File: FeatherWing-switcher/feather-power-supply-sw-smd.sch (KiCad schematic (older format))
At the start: 24 parts, among them J1 5.08mm, J2 Conn_01x12, J3 Conn_01x16, U1 TPS5405DR

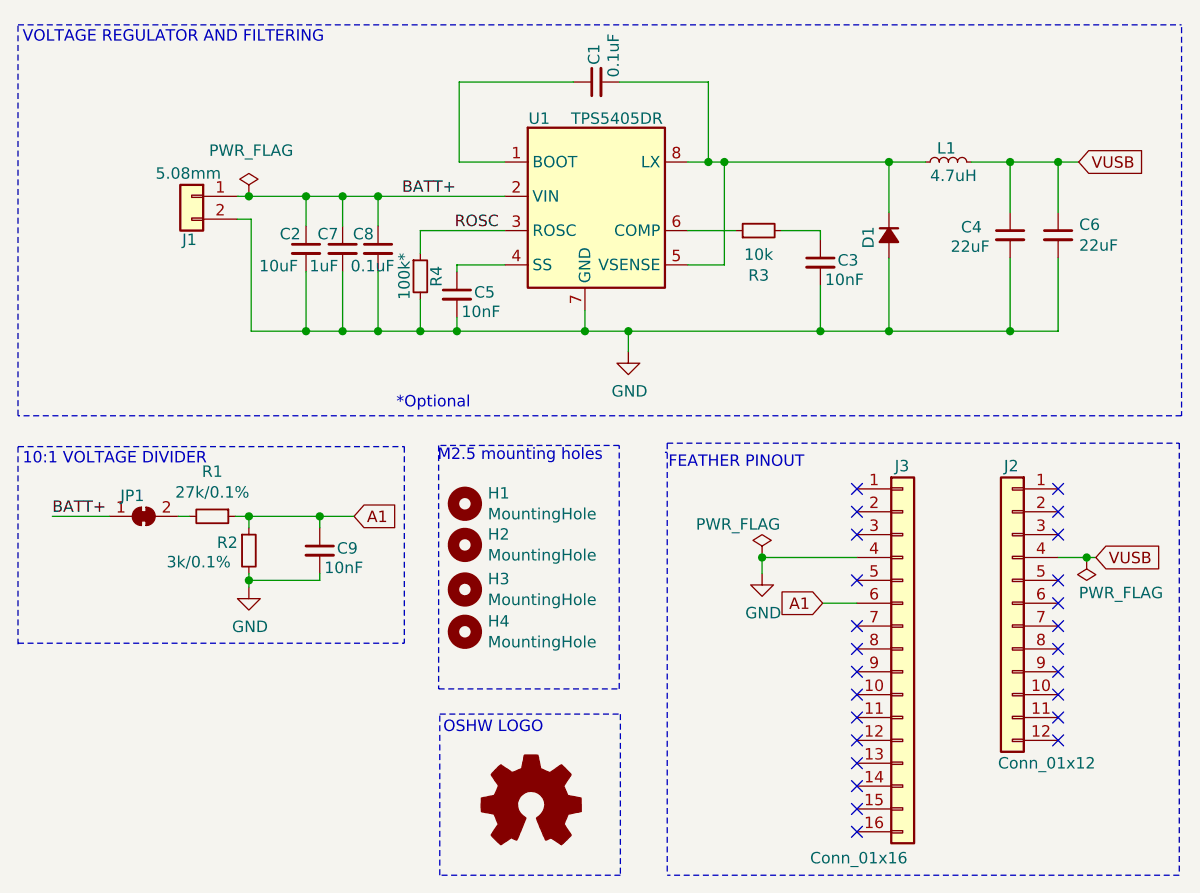
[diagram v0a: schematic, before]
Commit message: update mounting holes
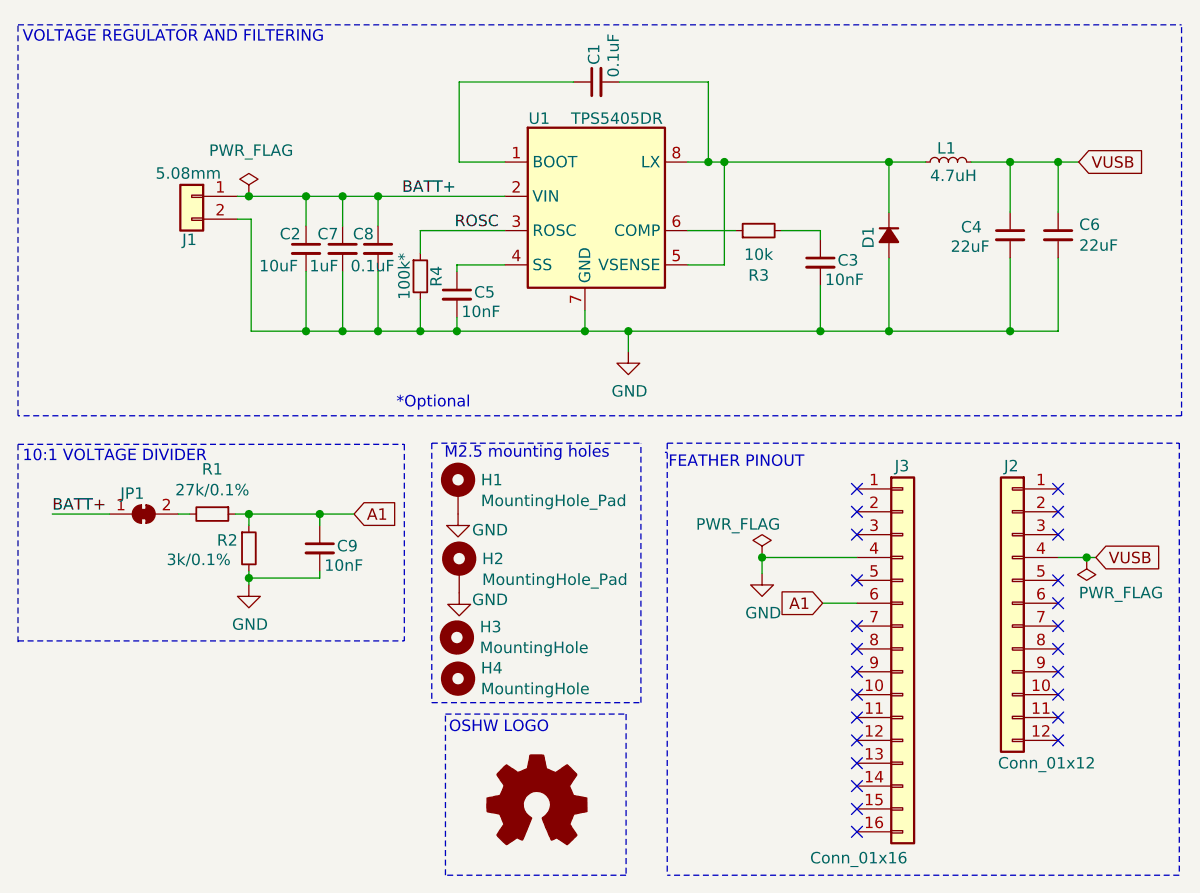
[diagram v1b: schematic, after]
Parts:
- removed H1, H2: MountingHole, MountingHole:MountingHole_2.7mm_M2.5, symbol Mechanical:MountingHole
- added H1, H2: MountingHole_Pad, MountingHole:MountingHole_2.5mm_Pad, symbol Mechanical:MountingHole_Pad
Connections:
- net GND: now also H1.1, H2.1
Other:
- moved on the sheet: H3, H4
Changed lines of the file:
@@
 $EndComp
 Connection ~ 6325 3900
-Text Label 3220 3720 0    50   ~ 0
+Text Label 3220 3710 0    50   ~ 0
 BATT+
-Text GLabel 4540 3720 2    50   Input ~ 0
+Text GLabel 4540 3710 2    50   Input ~ 0
 A1
 Text GLabel 6590 4100 0    50   Input ~ 0
@@
 	5910 3400 5910 5290
 Wire Notes Line
-	4760 3415 4760 4275
+	4760 3405 4760 4265
 Wire Notes Line
 	8160 1580 8160 3280
@@
 Wire Wire Line
 	4490 2910 4645 2910
-$Comp
-L Mechanical:MountingHole H1
-U 1 1 5F4DCA7B
-P 5025 3665
-F 0 "H1" H 5125 3711 50  0000 L CNN
-F 1 "MountingHole" H 5125 3620 50  0000 L CNN
-F 2 "MountingHole:MountingHole_2.7mm_M2.5" H 5025 3665 50  0001 C CNN
-F 3 "~" H 5025 3665 50  0001 C CNN
-	1    5025 3665
-	1    0    0    -1
-$EndComp
-$Comp
-L Mechanical:MountingHole H2
-U 1 1 5F4E3BF8
-P 5025 3845
-F 0 "H2" H 5125 3891 50  0000 L CNN
-F 1 "MountingHole" H 5125 3800 50  0000 L CNN
-F 2 "MountingHole:MountingHole_2.7mm_M2.5" H 5025 3845 50  0001 C CNN
-F 3 "~" H 5025 3845 50  0001 C CNN
-	1    5025 3845
-	1    0    0    -1
-$EndComp
-$Comp
-L Mechanical:MountingHole H3
-U 1 1 5F4E3ED4
-P 5025 4040
-F 0 "H3" H 5125 4086 50  0000 L CNN
-F 1 "MountingHole" H 5125 3995 50  0000 L CNN
-F 2 "MountingHole:MountingHole_2.7mm_M2.5" H 5025 4040 50  0001 C CNN
-F 3 "~" H 5025 4040 50  0001 C CNN
-	1    5025 4040
-	1    0    0    -1
-$EndComp
-$Comp
-L Mechanical:MountingHole H4
-U 1 1 5F4E4234
-P 5025 4225
-F 0 "H4" H 5125 4271 50  0000 L CNN
-F 1 "MountingHole" H 5125 4180 50  0000 L CNN
-F 2 "MountingHole:MountingHole_2.7mm_M2.5" H 5025 4225 50  0001 C CNN
-F 3 "~" H 5025 4225 50  0001 C CNN
-	1    5025 4225
-	1    0    0    -1
-$EndComp
-Wire Notes Line
-	4910 4475 5700 4475
-Wire Notes Line
-	5700 4475 5700 3410
-Wire Notes Line
-	5700 3410 4910 3410
-Wire Notes Line
-	4910 3410 4910 4475
-Text Notes 4905 3485 0    50   ~ 0
+Text Notes 4935 3475 0    50   ~ 0
 M2.5 mounting holes
 Wire Wire Line
-	3220 3720 3470 3720
-Wire Notes Line
-	3070 4275 4760 4275
-Wire Notes Line
-	3070 3415 4760 3415
-Wire Notes Line
-	3070 3415 3070 4280
+	3220 3710 3470 3710
+Wire Notes Line
+	3070 4265 4760 4265
+Wire Notes Line
+	3070 3405 4760 3405
+Wire Notes Line
+	3070 3405 3070 4270
 $Comp
 L Jumper:SolderJumper_2_Bridged JP1
 U 1 1 5F4E9F72
-P 3620 3720
-F 0 "JP1" H 3570 3810 50  0000 C CNN
-F 1 "SolderJumper_2_Bridged" H 3285 3630 50  0001 C CNN
-F 2 "Jumper:SolderJumper-2_P1.3mm_Bridged_RoundedPad1.0x1.5mm" H 3620 3720 50  0001 C CNN
-F 3 "~" H 3620 3720 50  0001 C CNN
-	1    3620 3720
-	1    0    0    -1
-$EndComp
-Text Notes 3090 3500 0    50   ~ 0
+P 3620 3710
+F 0 "JP1" H 3570 3800 50  0000 C CNN
+F 1 "SolderJumper_2_Bridged" H 3285 3620 50  0001 C CNN
+F 2 "Jumper:SolderJumper-2_P1.3mm_Bridged_RoundedPad1.0x1.5mm" H 3620 3710 50  0001 C CNN
+F 3 "~" H 3620 3710 50  0001 C CNN
+	1    3620 3710
+	1    0    0    -1
+$EndComp
+Text Notes 3090 3490 0    50   ~ 0
 10:1 VOLTAGE DIVIDER
 Wire Wire Line
-	4080 4030 4080 4000
-Wire Wire Line
-	4080 3720 4080 3770
+	4080 4020 4080 3990
+Wire Wire Line
+	4080 3710 4080 3760
 $Comp
 L power:GND #PWR02
 U 1 1 5F4755CE
-P 4080 4030
-F 0 "#PWR02" H 4080 3780 50  0001 C CNN
-F 1 "GND" H 4085 3857 50  0000 C CNN
-F 2 "" H 4080 4030 50  0001 C CNN
-F 3 "" H 4080 4030 50  0001 C CNN
-	1    4080 4030
+P 4080 4020
+F 0 "#PWR02" H 4080 3770 50  0001 C CNN
+F 1 "GND" H 4085 3847 50  0000 C CNN
+F 2 "" H 4080 4020 50  0001 C CNN
+F 3 "" H 4080 4020 50  0001 C CNN
+	1    4080 4020
 	1    0    0    -1
 $EndComp
@@
 L Device:R_Small R1
 U 1 1 5F47540B
-P 3920 3720
-F 0 "R1" V 3724 3720 50  0000 C CNN
-F 1 "27k/0.1%" V 3815 3720 50  0000 C CNN
-F 2 "Resistor_SMD:R_0603_1608Metric_Pad1.05x0.95mm_HandSolder" H 3920 3720 50  0001 C CNN
-F 3 "~" H 3920 3720 50  0001 C CNN
-F 4 "‎P20138CT-ND‎" V 3920 3720 50  0001 C CNN "DigiKey_PN"
-	1    3920 3720
+P 3920 3710
+F 0 "R1" V 3724 3710 50  0000 C CNN
+F 1 "27k/0.1%" V 3815 3710 50  0000 C CNN
+F 2 "Resistor_SMD:R_0603_1608Metric_Pad1.05x0.95mm_HandSolder" H 3920 3710 50  0001 C CNN
+F 3 "~" H 3920 3710 50  0001 C CNN
+F 4 "‎P20138CT-ND‎" V 3920 3710 50  0001 C CNN "DigiKey_PN"
+	1    3920 3710
 	0    1    1    0
 $EndComp
@@
 L Device:R_Small R2
 U 1 1 5F475325
-P 4080 3870
-F 0 "R2" H 3940 3905 50  0000 L CNN
-F 1 "3k/0.1%" H 3720 3820 50  0000 L CNN
-F 2 "Resistor_SMD:R_0603_1608Metric_Pad1.05x0.95mm_HandSolder" H 4080 3870 50  0001 C CNN
-F 3 "~" H 4080 3870 50  0001 C CNN
-F 4 "P20072CT-ND‎" H 4080 3870 50  0001 C CNN "DigiKey_PN"
-	1    4080 3870
+P 4080 3860
+F 0 "R2" H 3940 3895 50  0000 L CNN
+F 1 "3k/0.1%" H 3720 3810 50  0000 L CNN
+F 2 "Resistor_SMD:R_0603_1608Metric_Pad1.05x0.95mm_HandSolder" H 4080 3860 50  0001 C CNN
+F 3 "~" H 4080 3860 50  0001 C CNN
+F 4 "P20072CT-ND‎" H 4080 3860 50  0001 C CNN "DigiKey_PN"
+	1    4080 3860
 	1    0    0    -1
 $EndComp
@@
 $EndComp
 Wire Wire Line
-	3770 3720 3820 3720
+	3770 3710 3820 3710
 $Comp
 L Device:C_Small C9
 U 1 1 5F52B2E4
-P 4390 3870
-F 0 "C9" H 4465 3880 50  0000 L CNN
-F 1 "10nF" H 4410 3795 50  0000 L CNN
-F 2 "Capacitor_SMD:C_0603_1608Metric_Pad1.05x0.95mm_HandSolder" H 4390 3870 50  0001 C CNN
-F 3 "~" H 4390 3870 50  0001 C CNN
-	1    4390 3870
-	1    0    0    -1
-$EndComp
-Wire Wire Line
-	4540 3720 4390 3720
-Connection ~ 4080 3720
-Wire Wire Line
-	4080 3720 4020 3720
-Wire Wire Line
-	4390 3770 4390 3720
-Connection ~ 4390 3720
-Wire Wire Line
-	4390 3720 4080 3720
-Wire Wire Line
-	4390 3970 4390 4000
-Wire Wire Line
-	4390 4000 4080 4000
-Connection ~ 4080 4000
-Wire Wire Line
-	4080 4000 4080 3970
-$Comp
-L Graphic:Logo_Open_Hardware_Small #LOGO?
+P 4390 3860
+F 0 "C9" H 4465 3870 50  0000 L CNN
+F 1 "10nF" H 4410 3785 50  0000 L CNN
+F 2 "Capacitor_SMD:C_0603_1608Metric_Pad1.05x0.95mm_HandSolder" H 4390 3860 50  0001 C CNN
+F 3 "~" H 4390 3860 50  0001 C CNN
+	1    4390 3860
+	1    0    0    -1
+$EndComp
+Wire Wire Line
+	4540 3710 4390 3710
+Connection ~ 4080 3710
+Wire Wire Line
+	4080 3710 4020 3710
+Wire Wire Line
+	4390 3760 4390 3710
+Connection ~ 4390 3710
+Wire Wire Line
+	4390 3710 4080 3710
+Wire Wire Line
+	4390 3960 4390 3990
+Wire Wire Line
+	4390 3990 4080 3990
+Connection ~ 4080 3990
+Wire Wire Line
+	4080 3990 4080 3960
+$Comp
+L Graphic:Logo_Open_Hardware_Small #LOGO1
 U 1 1 5F51AA5B
-P 5315 4985
-F 0 "#LOGO?" H 5315 5260 50  0001 C CNN
-F 1 "Logo_Open_Hardware_Small" H 5315 4760 50  0001 C CNN
-F 2 "Symbol:OSHW-Logo2_7.3x6mm_Copper" H 5315 4985 50  0001 C CNN
-F 3 "~" H 5315 4985 50  0001 C CNN
-	1    5315 4985
-	1    0    0    -1
-$EndComp
-Wire Notes Line
-	5705 5290 4915 5290
-Wire Notes Line
-	4915 5290 4915 4585
-Wire Notes Line
-	4915 4585 5705 4585
-Wire Notes Line
-	5705 4585 5705 5290
-Text Notes 4930 4675 0    50   ~ 0
+P 5340 4985
+F 0 "#LOGO1" H 5340 5260 50  0001 C CNN
+F 1 "Logo_Open_Hardware_Small" H 5340 4760 50  0001 C CNN
+F 2 "Symbol:OSHW-Logo2_7.3x6mm_Copper" H 5340 4985 50  0001 C CNN
+F 3 "~" H 5340 4985 50  0001 C CNN
+	1    5340 4985
+	1    0    0    -1
+$EndComp
+Wire Notes Line
+	5730 5290 4940 5290
+Wire Notes Line
+	4940 5290 4940 4585
+Wire Notes Line
+	4940 4585 5730 4585
+Wire Notes Line
+	5730 4585 5730 5290
+Text Notes 4955 4675 0    50   ~ 0
 OSHW LOGO
+$Comp
+L Mechanical:MountingHole H4
+U 1 1 5F4E4234
+P 4995 4430
+F 0 "H4" H 5095 4476 50  0000 L CNN
+F 1 "MountingHole" H 5095 4385 50  0000 L CNN
+F 2 "MountingHole:MountingHole_2.7mm_M2.5" H 4995 4430 50  0001 C CNN
+F 3 "~" H 4995 4430 50  0001 C CNN
+	1    4995 4430
+	1    0    0    -1
+$EndComp
+$Comp
+L Mechanical:MountingHole_Pad H1
+U 1 1 5F541A68
+P 4995 3610
+F 0 "H1" H 5095 3659 50  0000 L CNN
+F 1 "MountingHole_Pad" H 5095 3568 50  0000 L CNN
+F 2 "MountingHole:MountingHole_2.5mm_Pad" H 4995 3610 50  0001 C CNN
+F 3 "~" H 4995 3610 50  0001 C CNN
+	1    4995 3610
+	1    0    0    -1
+$EndComp
+$Comp
+L Mechanical:MountingHole H3
+U 1 1 5F4E3ED4
+P 4990 4250
+F 0 "H3" H 5090 4296 50  0000 L CNN
+F 1 "MountingHole" H 5090 4205 50  0000 L CNN
+F 2 "MountingHole:MountingHole_2.7mm_M2.5" H 4990 4250 50  0001 C CNN
+F 3 "~" H 4990 4250 50  0001 C CNN
+	1    4990 4250
+	1    0    0    -1
+$EndComp
+$Comp
+L Mechanical:MountingHole_Pad H2
+U 1 1 5F54DC92
+P 5000 3955
+F 0 "H2" H 5100 4004 50  0000 L CNN
+F 1 "MountingHole_Pad" H 5100 3913 50  0000 L CNN
+F 2 "MountingHole:MountingHole_2.5mm_Pad" H 5000 3955 50  0001 C CNN
+F 3 "~" H 5000 3955 50  0001 C CNN
+	1    5000 3955
+	1    0    0    -1
+$EndComp
+$Comp
+L power:GND #PWR04
+U 1 1 5F54E691
+P 4995 3710
+F 0 "#PWR04" H 4995 3460 50  0001 C CNN
+F 1 "GND" H 5135 3640 50  0000 C CNN
+F 2 "" H 4995 3710 50  0001 C CNN
+F 3 "" H 4995 3710 50  0001 C CNN
+	1    4995 3710
+	1    0    0    -1
+$EndComp
+$Comp
+L power:GND #PWR05
+U 1 1 5F55451D
+P 5000 4055
+F 0 "#PWR05" H 5000 3805 50  0001 C CNN
+F 1 "GND" H 5135 4025 50  0000 C CNN
+F 2 "" H 5000 4055 50  0001 C CNN
+F 3 "" H 5000 4055 50  0001 C CNN
+	1    5000 4055
+	1    0    0    -1
+$EndComp
+Wire Notes Line
+	4880 4535 5795 4535
+Wire Notes Line
+	5795 4535 5795 3400
+Wire Notes Line
+	4880 3400 5795 3400
+Wire Notes Line
+	4880 3400 4880 4535
 $EndSCHEMATC
